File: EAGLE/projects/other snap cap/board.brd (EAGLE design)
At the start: 139.7 x 64.4 mm, 6 parts

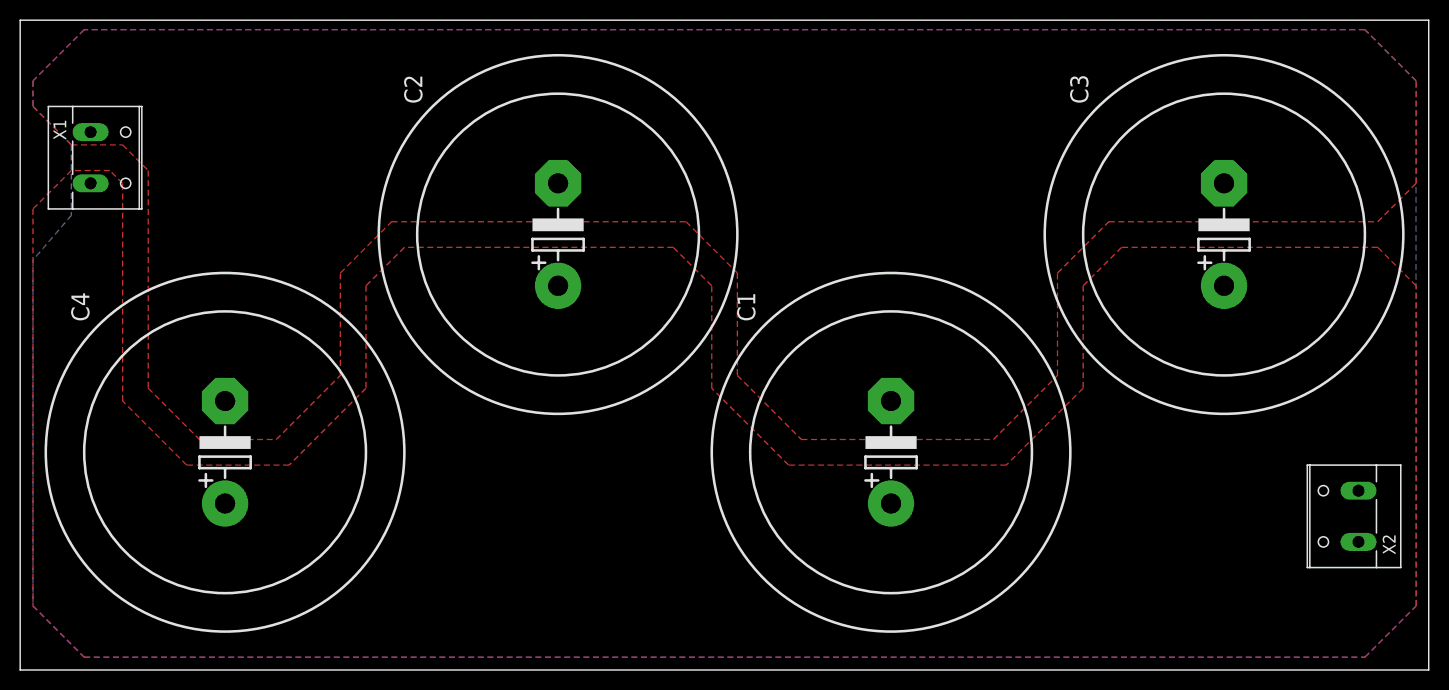
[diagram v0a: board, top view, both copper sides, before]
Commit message: PS
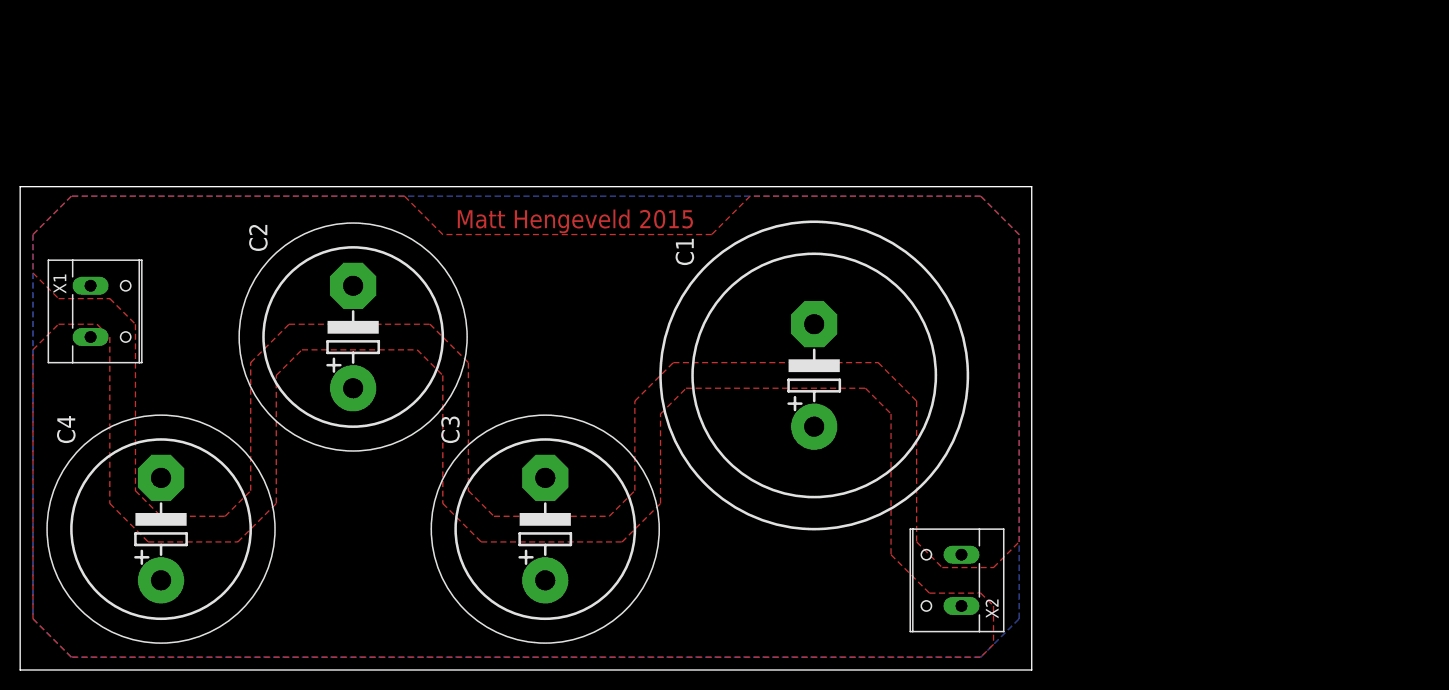
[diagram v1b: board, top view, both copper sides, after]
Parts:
- C1: device rcl:EB35D -> rcl:EB30D
- C2, C3, C4: device rcl:EB35D -> rcl:EB22,5D
- moved C3 73.4 mm to (52.1, 14.0)
- moved X2 39.9 mm to (92.7, 8.89)
- moved C2 22.7 mm to (33.0, 33.0)
- moved X1 15.2 mm to (7.62, 35.6)
- moved C1 10.8 mm to (78.7, 29.2)
- moved C4 9.92 mm to (14.0, 14.0)
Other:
- board size 139.7 x 64.4 mm -> 100.3 x 47.9 mm
- board text added: "Matt Hengeveld 2015"
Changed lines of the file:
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@@
 <board>
 <plain>
-<wire x1="0" y1="0" x2="139.68" y2="0" width="0" layer="20"/>
-<wire x1="139.68" y1="0" x2="139.68" y2="64.44" width="0" layer="20"/>
-<wire x1="139.68" y1="64.44" x2="0" y2="64.44" width="0" layer="20"/>
-<wire x1="0" y1="64.44" x2="0" y2="0" width="0" layer="20"/>
+<wire x1="0" y1="0" x2="100.31" y2="0" width="0" layer="20"/>
+<wire x1="100.31" y1="0" x2="100.31" y2="47.93" width="0" layer="20"/>
+<wire x1="100.31" y1="47.93" x2="0" y2="47.93" width="0" layer="20"/>
+<wire x1="0" y1="47.93" x2="0" y2="0" width="0" layer="20"/>
+<text x="43.18" y="43.815" size="1.778" layer="1">Matt Hengeveld 2015</text>
 </plain>
 <attributes>
@@
 </autorouter>
 <elements>
-<element name="C1" library="rcl" package="EB35D" value="" x="86.36" y="21.59" rot="R90"/>
-<element name="C2" library="rcl" package="EB35D" value="" x="53.34" y="43.18" rot="R90"/>
-<element name="C3" library="rcl" package="EB35D" value="" x="119.38" y="43.18" rot="R90"/>
-<element name="C4" library="rcl" package="EB35D" value="" x="20.32" y="21.59" rot="R90"/>
-<element name="X1" library="con-wago-508" package="W237-132" value="" x="7.62" y="50.8" rot="R270">
-<attribute name="OC_NEWARK" value="unknown" x="7.62" y="50.8" size="1.778" layer="27" rot="R270" display="off"/>
-<attribute name="MPN" value="" x="7.62" y="50.8" size="1.778" layer="27" rot="R270" display="off"/>
-<attribute name="MF" value="" x="7.62" y="50.8" size="1.778" layer="27" rot="R270" display="off"/>
-<attribute name="OC_FARNELL" value="unknown" x="7.62" y="50.8" size="1.778" layer="27" rot="R270" display="off"/>
+<element name="C1" library="rcl" package="EB30D" value="" x="78.74" y="29.21" rot="R90"/>
+<element name="C2" library="rcl" package="EB22,5D" value="" x="33.02" y="33.02" rot="R90"/>
+<element name="C3" library="rcl" package="EB22,5D" value="" x="52.07" y="13.97" rot="R90"/>
+<element name="C4" library="rcl" package="EB22,5D" value="" x="13.97" y="13.97" rot="R90"/>
+<element name="X1" library="con-wago-508" package="W237-132" value="" x="7.62" y="35.56" rot="R270">
+<attribute name="OC_NEWARK" value="unknown" x="7.62" y="35.56" size="1.778" layer="27" rot="R270" display="off"/>
+<attribute name="MPN" value="" x="7.62" y="35.56" size="1.778" layer="27" rot="R270" display="off"/>
+<attribute name="MF" value="" x="7.62" y="35.56" size="1.778" layer="27" rot="R270" display="off"/>
+<attribute name="OC_FARNELL" value="unknown" x="7.62" y="35.56" size="1.778" layer="27" rot="R270" display="off"/>
 </element>
-<element name="X2" library="con-wago-508" package="W237-132" value="" x="132.08" y="15.24" rot="R90">
-<attribute name="OC_NEWARK" value="unknown" x="132.08" y="15.24" size="1.778" layer="27" rot="R90" display="off"/>
-<attribute name="MPN" value="" x="132.08" y="15.24" size="1.778" layer="27" rot="R90" display="off"/>
-<attribute name="MF" value="" x="132.08" y="15.24" size="1.778" layer="27" rot="R90" display="off"/>
-<attribute name="OC_FARNELL" value="unknown" x="132.08" y="15.24" size="1.778" layer="27" rot="R90" display="off"/>
+<element name="X2" library="con-wago-508" package="W237-132" value="" x="92.71" y="8.89" rot="R90">
+<attribute name="OC_NEWARK" value="unknown" x="92.71" y="8.89" size="1.778" layer="27" rot="R90" display="off"/>
+<attribute name="MPN" value="" x="92.71" y="8.89" size="1.778" layer="27" rot="R90" display="off"/>
+<attribute name="MF" value="" x="92.71" y="8.89" size="1.778" layer="27" rot="R90" display="off"/>
+<attribute name="OC_FARNELL" value="unknown" x="92.71" y="8.89" size="1.778" layer="27" rot="R90" display="off"/>
 </element>
 </elements>
 <signals>
 <signal name="GND">
-<polygon width="0.4064" layer="16" isolate="2.54" thermals="no">
-<vertex x="133.35" y="63.5"/>
-<vertex x="6.35" y="63.5"/>
-<vertex x="1.27" y="58.42"/>
-<vertex x="1.27" y="55.88"/>
-<vertex x="5.08" y="52.07"/>
-<vertex x="5.08" y="45.085"/>
-<vertex x="1.27" y="40.64"/>
-<vertex x="1.27" y="6.35"/>
-<vertex x="6.35" y="1.27"/>
-<vertex x="133.35" y="1.27"/>
-<vertex x="138.43" y="6.35"/>
-<vertex x="138.43" y="58.42"/>
-</polygon>
-<polygon width="0.4064" layer="1" isolate="1.6764" thermals="no">
-<vertex x="6.35" y="63.5"/>
-<vertex x="1.27" y="58.42"/>
-<vertex x="1.27" y="55.88"/>
-<vertex x="5.08" y="52.07"/>
-<vertex x="10.16" y="52.07"/>
-<vertex x="12.7" y="49.53"/>
-<vertex x="12.7" y="27.94"/>
-<vertex x="17.78" y="22.86"/>
-<vertex x="25.4" y="22.86"/>
-<vertex x="31.75" y="29.21"/>
-<vertex x="31.75" y="39.37"/>
-<vertex x="36.83" y="44.45"/>
-<vertex x="66.04" y="44.45"/>
-<vertex x="71.12" y="39.37"/>
-<vertex x="71.12" y="29.21"/>
-<vertex x="77.47" y="22.86"/>
-<vertex x="96.52" y="22.86"/>
-<vertex x="102.87" y="29.21"/>
-<vertex x="102.87" y="39.37"/>
-<vertex x="107.95" y="44.45"/>
-<vertex x="134.62" y="44.45"/>
-<vertex x="138.43" y="48.26"/>
-<vertex x="138.43" y="58.42"/>
-<vertex x="133.35" y="63.5"/>
-</polygon>
 <contactref element="C1" pad="-"/>
 <contactref element="C4" pad="-"/>
@@
 <contactref element="X1" pad="1"/>
 <contactref element="X2" pad="2"/>
+<polygon width="0.4064" layer="1" thermals="no">
+<vertex x="5.08" y="46.99"/>
+<vertex x="1.27" y="43.18"/>
+<vertex x="1.27" y="39.37"/>
+<vertex x="3.81" y="36.83"/>
+<vertex x="8.89" y="36.83"/>
+<vertex x="11.43" y="34.29"/>
+<vertex x="11.43" y="17.78"/>
+<vertex x="13.97" y="15.24"/>
+<vertex x="20.32" y="15.24"/>
+<vertex x="22.86" y="17.78"/>
+<vertex x="22.86" y="30.48"/>
+<vertex x="26.67" y="34.29"/>
+<vertex x="40.64" y="34.29"/>
+<vertex x="44.45" y="30.48"/>
+<vertex x="44.45" y="17.78"/>
+<vertex x="46.99" y="15.24"/>
+<vertex x="58.42" y="15.24"/>
+<vertex x="60.96" y="17.78"/>
+<vertex x="60.96" y="26.67"/>
+<vertex x="64.77" y="30.48"/>
+<vertex x="85.09" y="30.48"/>
+<vertex x="88.9" y="26.67"/>
+<vertex x="88.9" y="12.7"/>
+<vertex x="91.44" y="10.16"/>
+<vertex x="96.52" y="10.16"/>
+<vertex x="99.06" y="12.7"/>
+<vertex x="99.06" y="43.18"/>
+<vertex x="95.25" y="46.99"/>
+<vertex x="72.39" y="46.99"/>
+<vertex x="68.58" y="43.18"/>
+<vertex x="41.91" y="43.18"/>
+<vertex x="38.1" y="46.99"/>
+</polygon>
+<polygon width="0.4064" layer="16" isolate="1.6764">
+<vertex x="95.25" y="46.99"/>
+<vertex x="5.08" y="46.99"/>
+<vertex x="1.27" y="43.18"/>
+<vertex x="1.27" y="5.08"/>
+<vertex x="5.08" y="1.27"/>
+<vertex x="95.25" y="1.27"/>
+<vertex x="99.06" y="5.08"/>
+<vertex x="99.06" y="43.18"/>
+</polygon>
 </signal>
 <signal name="V+">
-<polygon width="0.4064" layer="1" isolate="1.778" thermals="no">
-<vertex x="5.08" y="49.53"/>
-<vertex x="1.27" y="45.72"/>
-<vertex x="1.27" y="6.35"/>
-<vertex x="6.35" y="1.27"/>
-<vertex x="133.35" y="1.27"/>
-<vertex x="138.43" y="6.35"/>
-<vertex x="138.43" y="38.1"/>
-<vertex x="134.62" y="41.91"/>
-<vertex x="109.22" y="41.91"/>
-<vertex x="105.41" y="38.1"/>
-<vertex x="105.41" y="27.94"/>
-<vertex x="97.79" y="20.32"/>
-<vertex x="76.2" y="20.32"/>
-<vertex x="68.58" y="27.94"/>
-<vertex x="68.58" y="38.1"/>
-<vertex x="64.77" y="41.91"/>
-<vertex x="38.1" y="41.91"/>
-<vertex x="34.29" y="38.1"/>
-<vertex x="34.29" y="27.94"/>
-<vertex x="26.67" y="20.32"/>
-<vertex x="16.51" y="20.32"/>
-<vertex x="10.16" y="26.67"/>
-<vertex x="10.16" y="48.26"/>
-<vertex x="8.89" y="49.53"/>
-</polygon>
 <contactref element="C1" pad="+"/>
 <contactref element="C4" pad="+"/>
@@
 <contactref element="X1" pad="2"/>
 <contactref element="X2" pad="1"/>
+<polygon width="0.4064" layer="1" thermals="no">
+<vertex x="1.27" y="31.75"/>
+<vertex x="3.81" y="34.29"/>
+<vertex x="7.62" y="34.29"/>
+<vertex x="8.89" y="33.02"/>
+<vertex x="8.89" y="16.51"/>
+<vertex x="12.7" y="12.7"/>
+<vertex x="21.59" y="12.7"/>
+<vertex x="25.4" y="16.51"/>
+<vertex x="25.4" y="29.21"/>
+<vertex x="27.94" y="31.75"/>
+<vertex x="39.37" y="31.75"/>
+<vertex x="41.91" y="29.21"/>
+<vertex x="41.91" y="16.51"/>
+<vertex x="45.72" y="12.7"/>
+<vertex x="59.69" y="12.7"/>
+<vertex x="63.5" y="16.51"/>
+<vertex x="63.5" y="25.4"/>
+<vertex x="66.04" y="27.94"/>
+<vertex x="83.82" y="27.94"/>
+<vertex x="86.36" y="25.4"/>
+<vertex x="86.36" y="11.43"/>
+<vertex x="90.17" y="7.62"/>
+<vertex x="95.25" y="7.62"/>
+<vertex x="96.52" y="6.35"/>
+<vertex x="96.52" y="2.54"/>
+<vertex x="95.25" y="1.27"/>
+<vertex x="5.08" y="1.27"/>
+<vertex x="1.27" y="5.08"/>
+</polygon>
 </signal>
 </signals>
